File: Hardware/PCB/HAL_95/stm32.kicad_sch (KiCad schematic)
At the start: 25 parts, among them J1 ST_LINK, J3 NEOPIXELS, SW1 USER_BTN, SW2 NRST, U1 STM32G431RBTx, U6 SN74AHCT1G125DBVR, Y1 16MHz

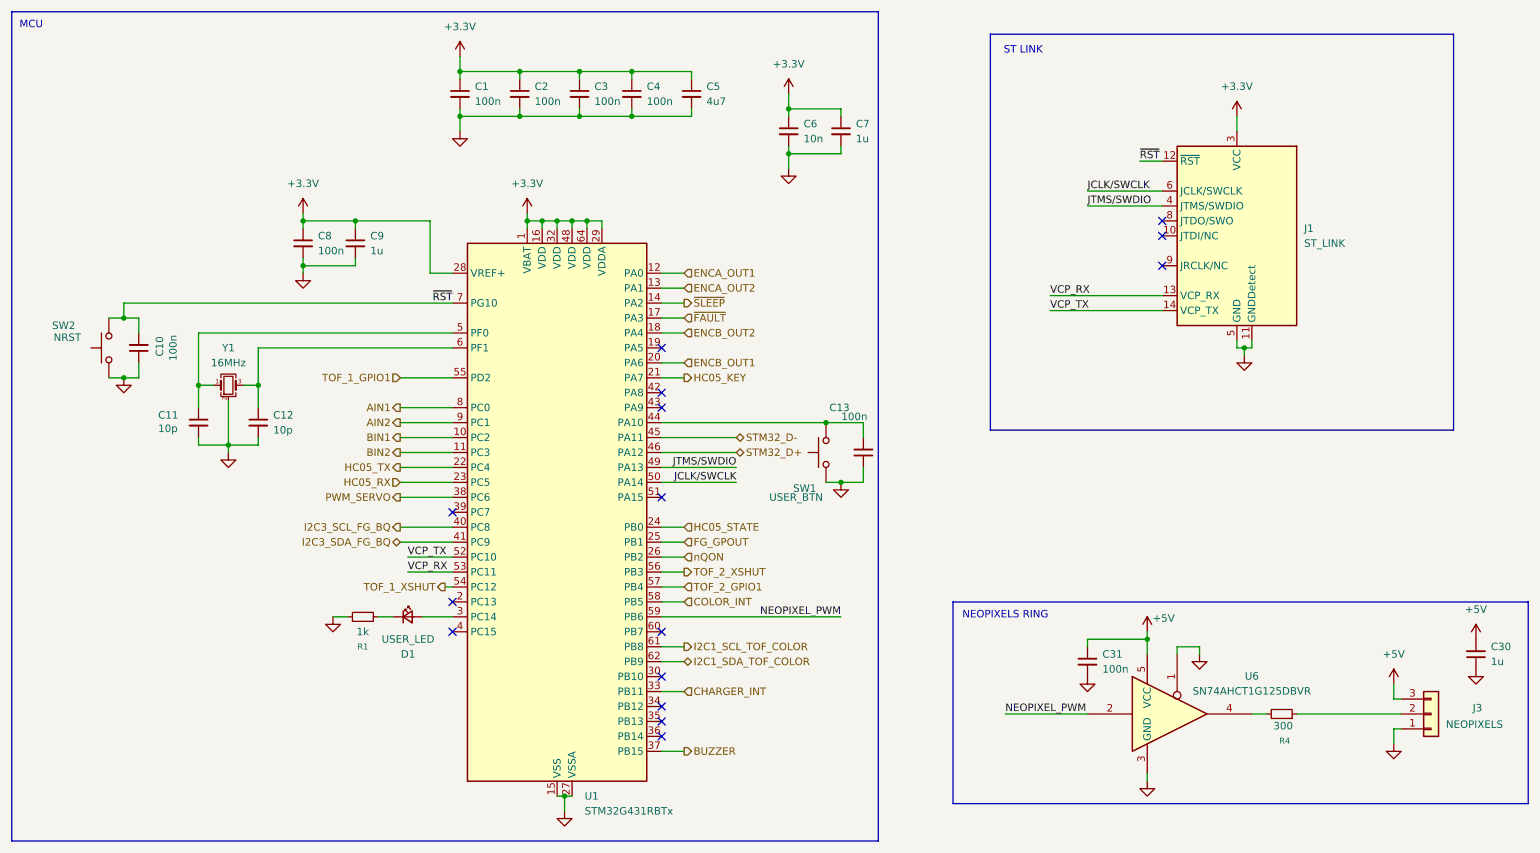
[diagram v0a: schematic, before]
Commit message: enhanced routing
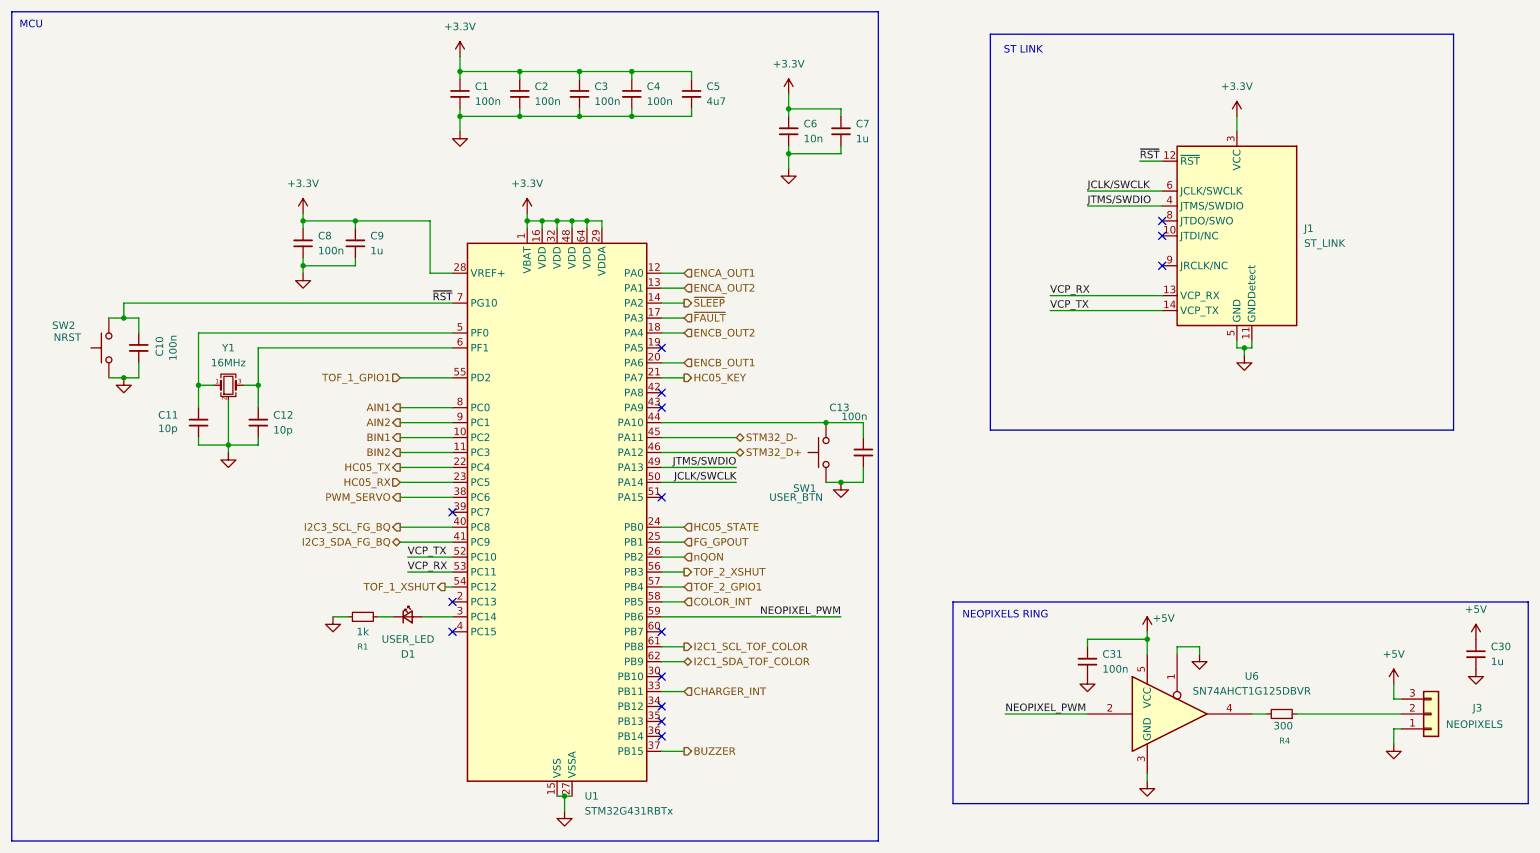
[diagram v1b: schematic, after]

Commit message: added logo
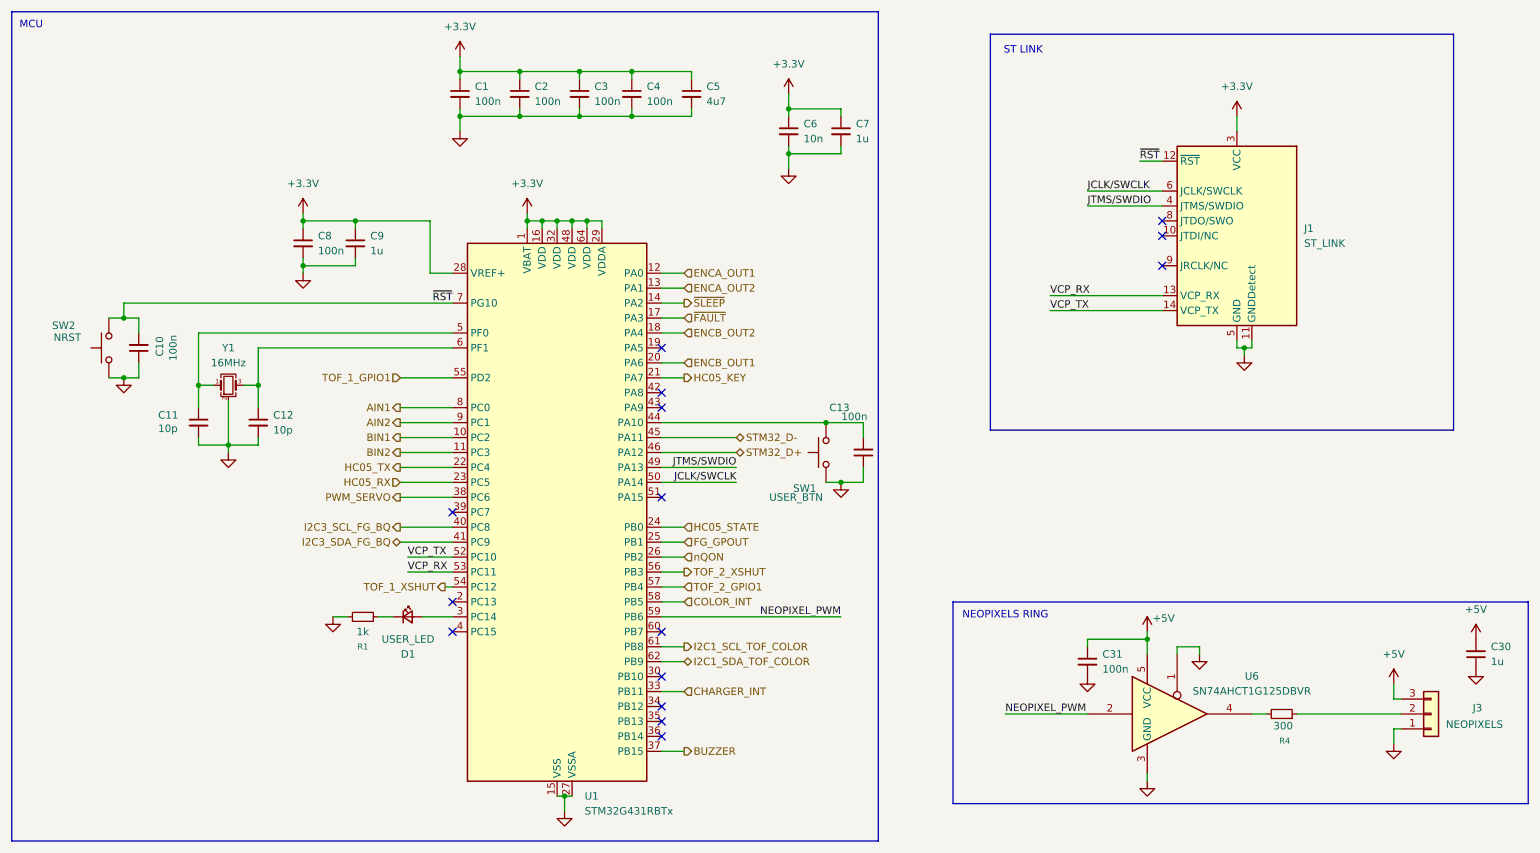
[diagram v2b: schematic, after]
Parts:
- R4: JLCPCB Part # C23025 -> C23025
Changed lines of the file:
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@@
 			)
 		)
-		(property "JLCPCB Part #" " C23025"
+		(property "JLCPCB Part #" "C23025"
 			(at 240.03 147.32 90)
 			(hide yes)
